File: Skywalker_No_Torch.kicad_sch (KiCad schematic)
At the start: 42 parts

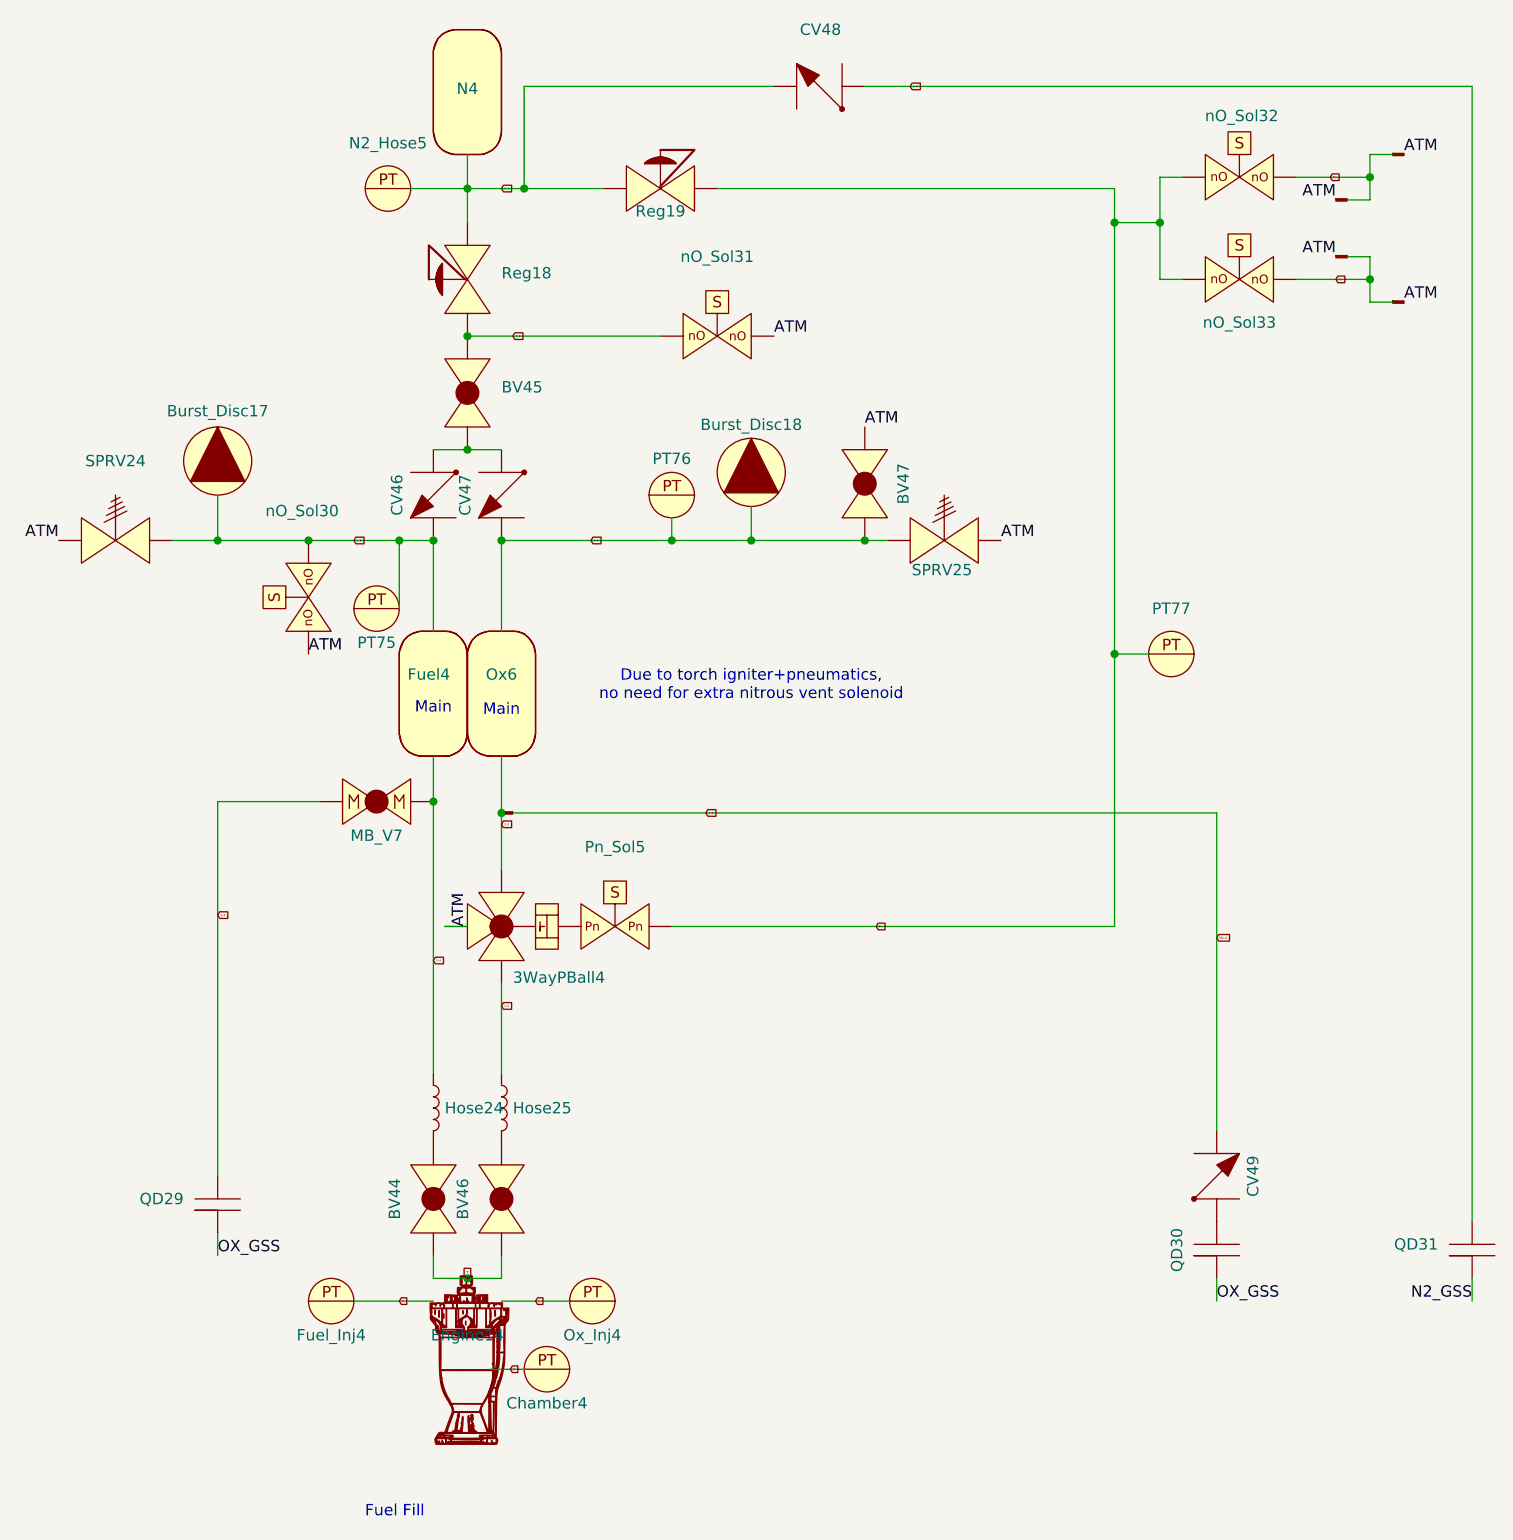
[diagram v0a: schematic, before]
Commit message: j0
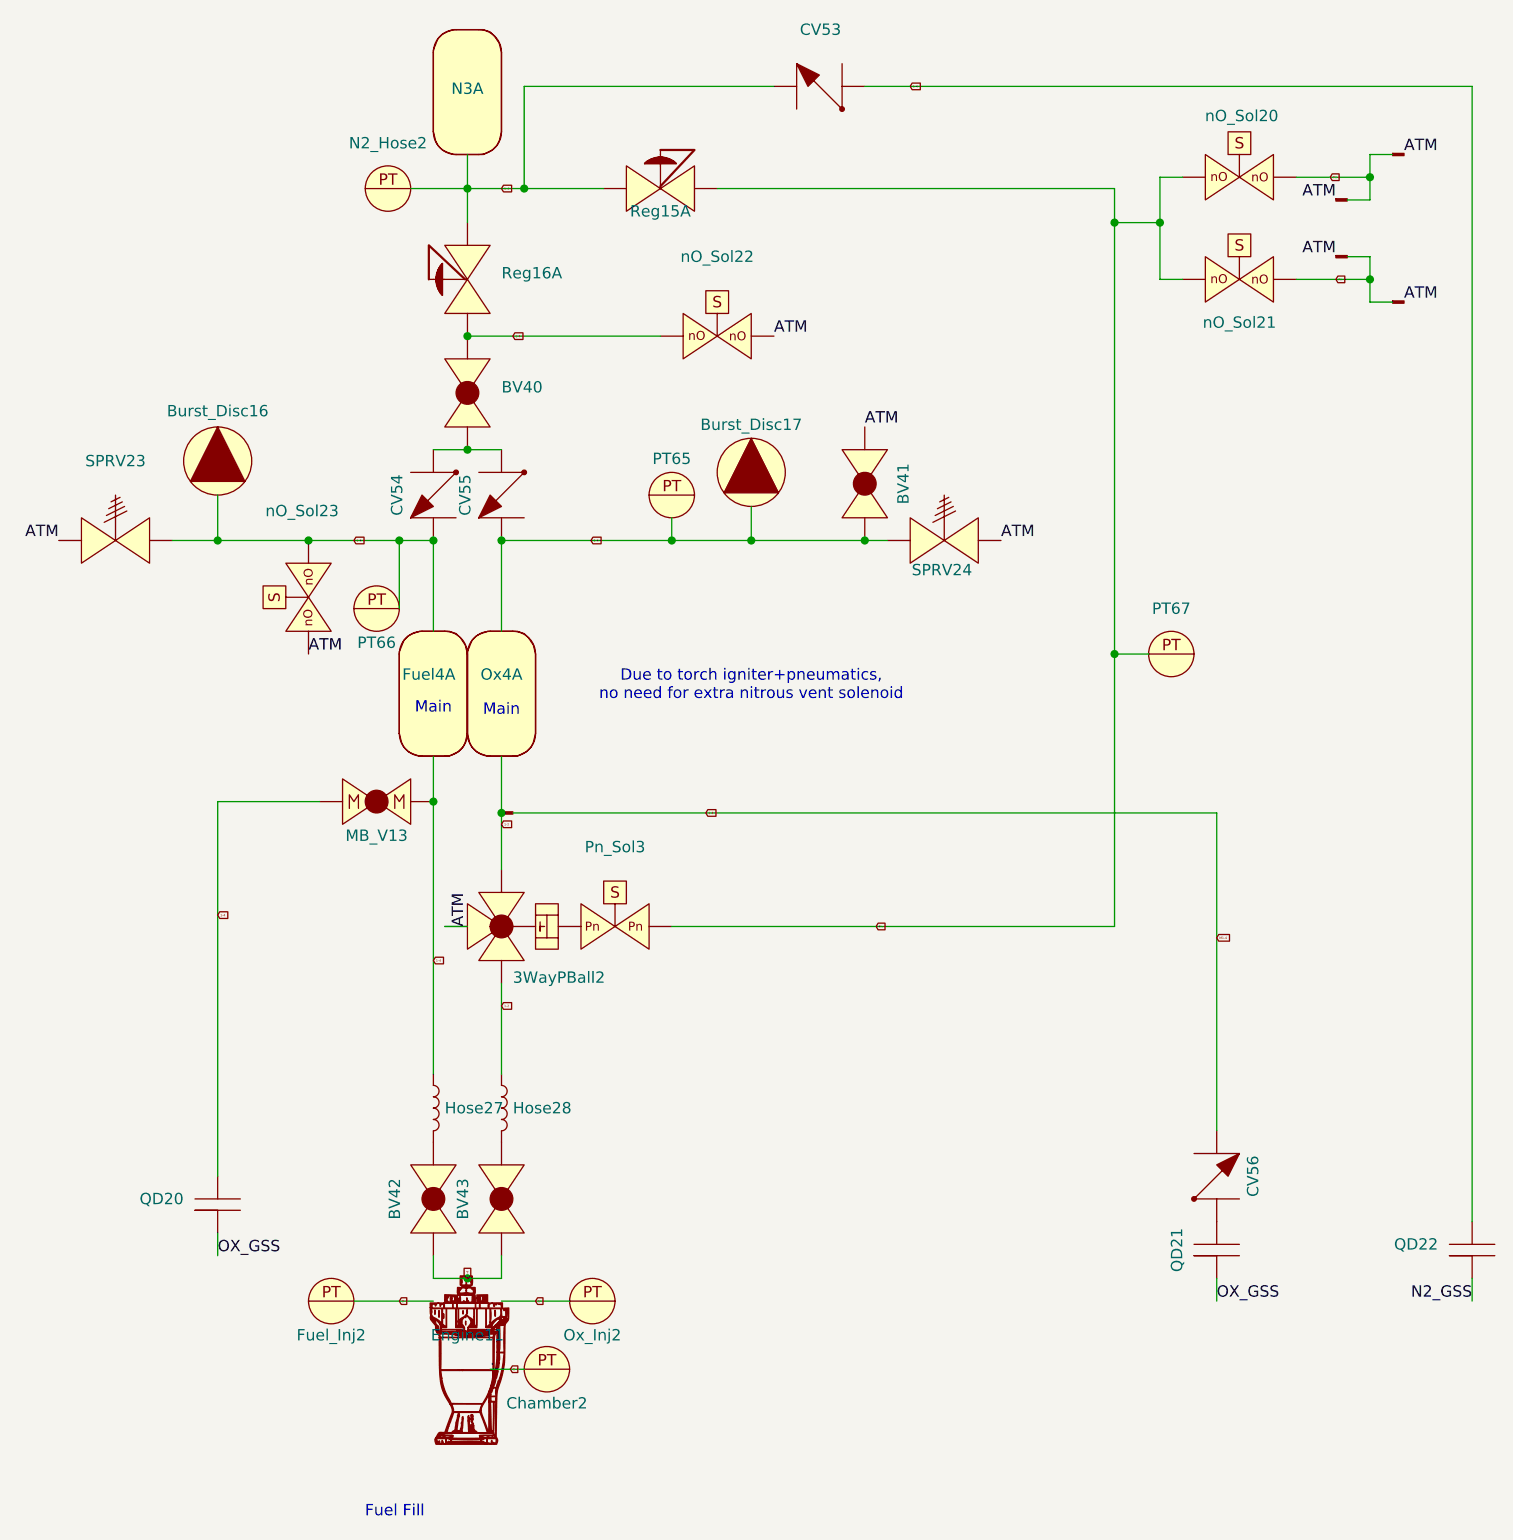
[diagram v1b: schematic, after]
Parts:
- renumbered 3WayPBall4 to 3WayPBall2, BV45 to BV40, BV47 to BV41, BV44 to BV42, BV46 to BV43, Burst_Disc17 to Burst_Disc16, Burst_Disc18 to Burst_Disc17, CV48 to CV53, CV46 to CV54, CV47 to CV55, CV49 to CV56, Chamber4 to Chamber2, Engine14 to Engine11, Fuel_Inj4 to Fuel_Inj2, Hose24 to Hose27, Hose25 to Hose28, MB_V7 to MB_V13, N2_Hose5 to N2_Hose2, N4 to N3, Ox6 to Ox4, Ox_Inj4 to Ox_Inj2, PT76 to PT65, PT75 to PT66, PT77 to PT67, Pn_Sol5 to Pn_Sol3, QD29 to QD20, QD30 to QD21, QD31 to QD22, Reg19 to Reg15, Reg18 to Reg16, SPRV24 to SPRV23, SPRV25 to SPRV24, U45 to U48, U46 to U49, U48 to U50, U44 to U51, nO_Sol32 to nO_Sol20, nO_Sol33 to nO_Sol21, nO_Sol31 to nO_Sol22, nO_Sol30 to nO_Sol23
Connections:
- new net: BV40., CV54., CV55.
- new net: CV56., QD21.
- new net: 3WayPBall2., Pn_Sol3.

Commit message: more silwood stuff
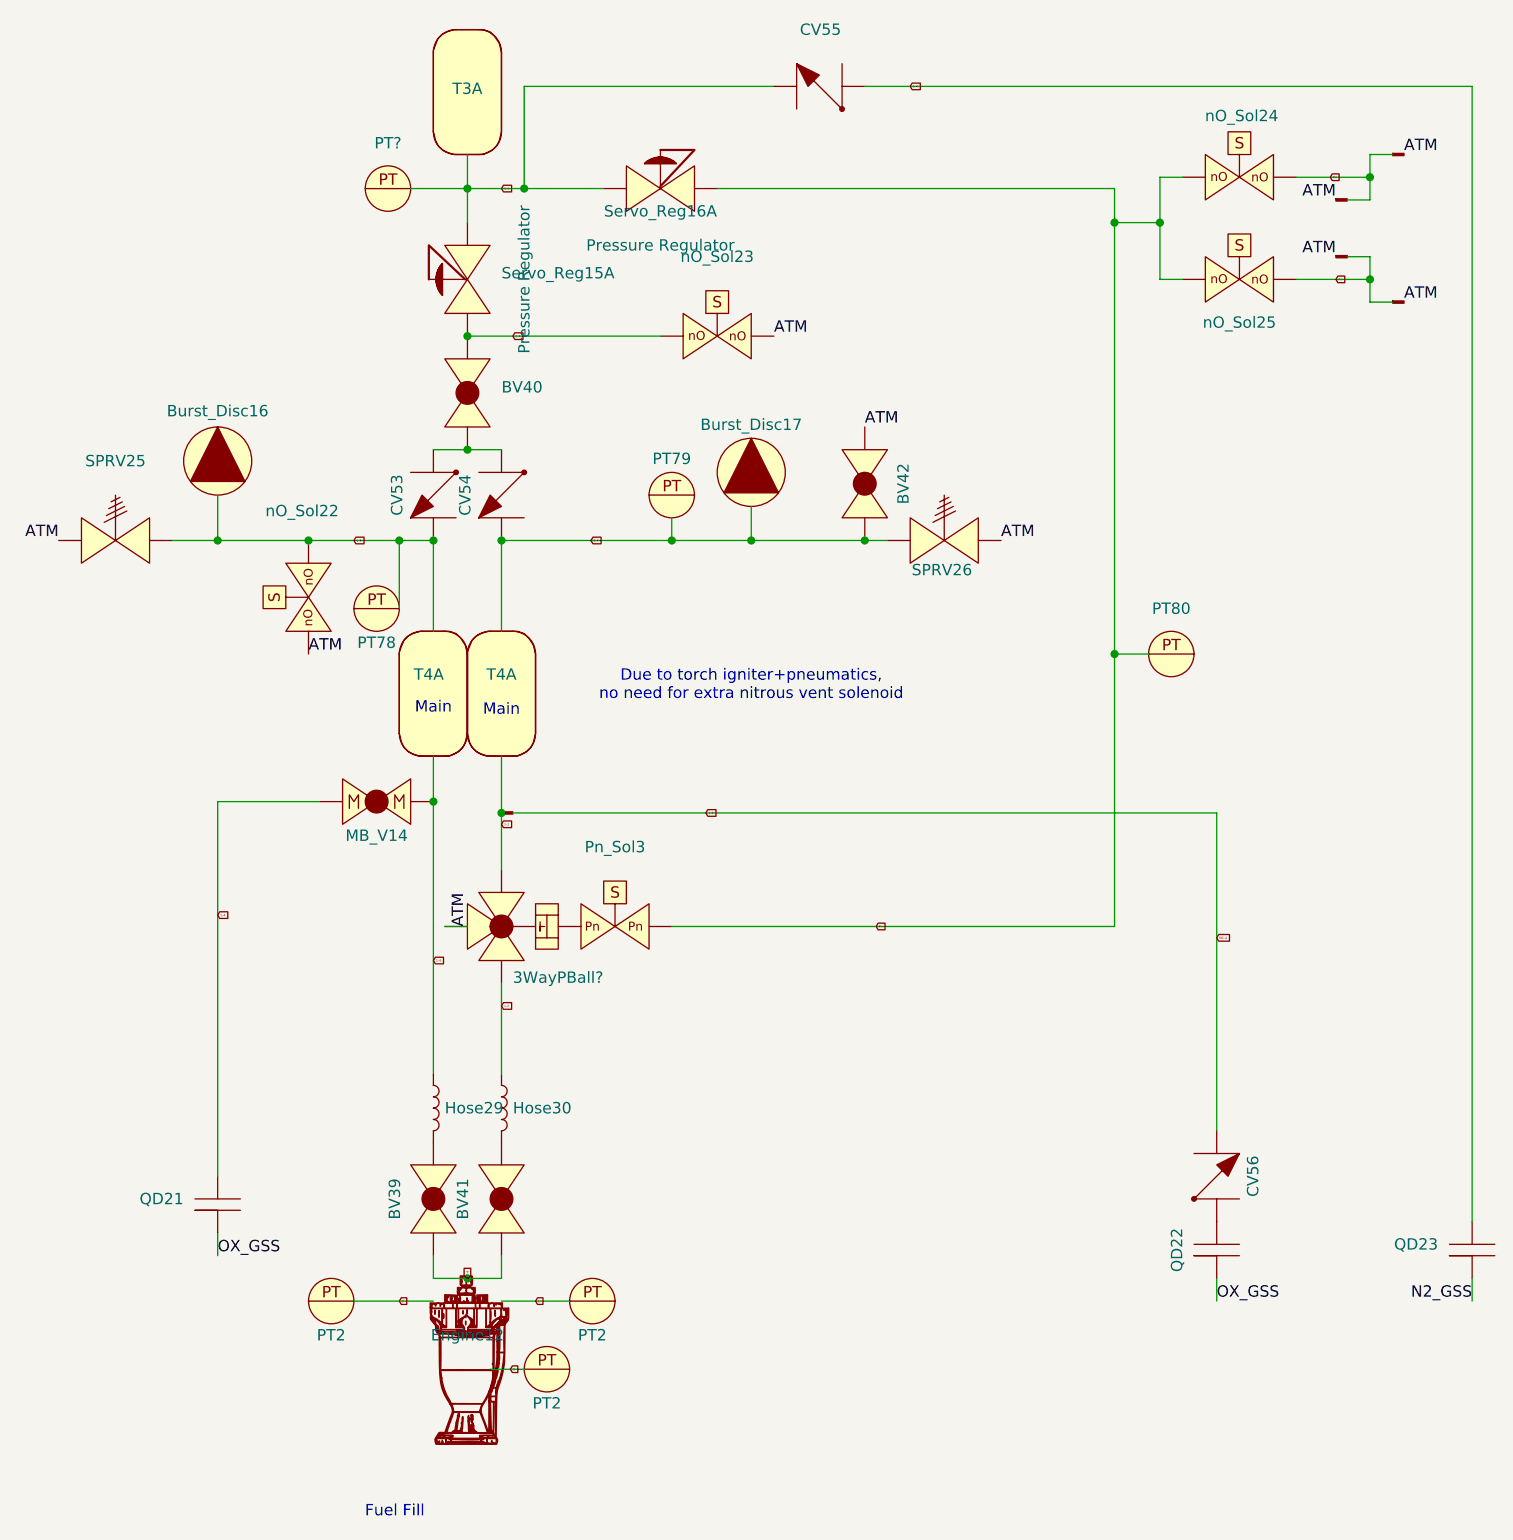
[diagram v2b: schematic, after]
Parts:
- renumbered 3WayPBall2 to 3WayPBall?, BV42 to BV39, BV43 to BV41, BV41 to BV42, CV54 to CV53, CV55 to CV54, CV53 to CV55, Engine11 to Engine12, Hose27 to Hose29, Hose28 to Hose30, MB_V13 to MB_V14, Chamber2 to PT2, Ox_Inj2 to PT2, Fuel_Inj2 to PT2, PT66 to PT78, PT65 to PT79, PT67 to PT80, N2_Hose2 to PT?, QD20 to QD21, QD21 to QD22, QD22 to QD23, SPRV23 to SPRV25, SPRV24 to SPRV26, Reg16 to Servo_Reg15, Reg15 to Servo_Reg16, N3 to T3, Fuel4 to T4, Ox4 to T4, U51 to U62, U48 to U63, U49 to U64, U47 to U65, U50 to U66, nO_Sol23 to nO_Sol22, nO_Sol22 to nO_Sol23, nO_Sol20 to nO_Sol24, nO_Sol21 to nO_Sol25
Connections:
- new net: BV40., CV53., CV54.
- new net: CV56., QD22.
- new net: 3WayPBall?., Pn_Sol3.

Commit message: Formatiing
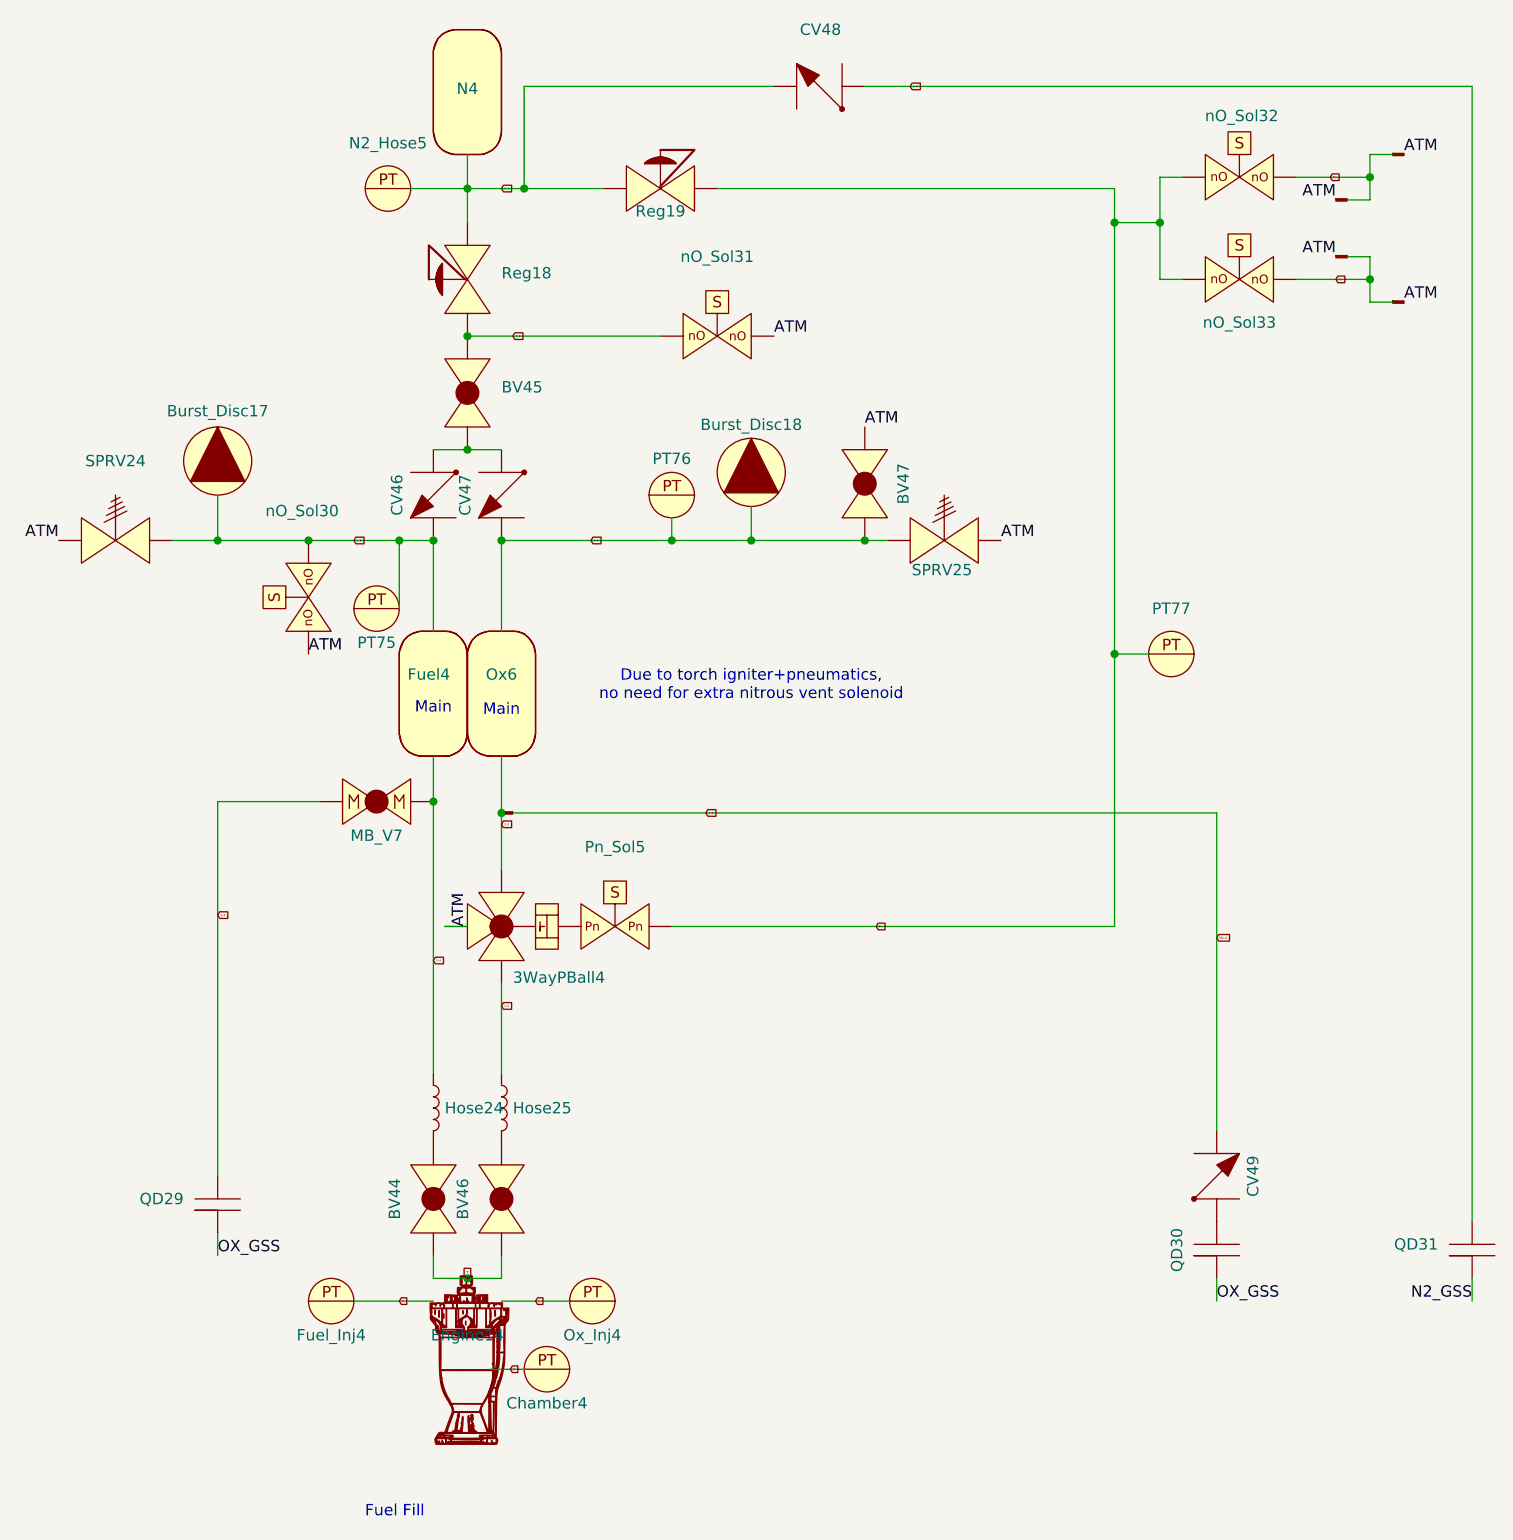
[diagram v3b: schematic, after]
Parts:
- gave numbers to parts that had none: 2
- renumbered BV39 to BV44, BV40 to BV45, BV41 to BV46, BV42 to BV47, Burst_Disc16 to Burst_Disc17, Burst_Disc17 to Burst_Disc18, CV53 to CV46, CV54 to CV47, CV55 to CV48, CV56 to CV49, PT2 to Chamber4, Engine12 to Engine14, T4 to Fuel4, PT2 to Fuel_Inj4, Hose29 to Hose24, Hose30 to Hose25, MB_V14 to MB_V7, T3 to N4, T4 to Ox6, PT2 to Ox_Inj4, PT78 to PT75, PT79 to PT76, PT80 to PT77, Pn_Sol3 to Pn_Sol5, QD21 to QD29, QD22 to QD30, QD23 to QD31, Servo_Reg15 to Reg18, Servo_Reg16 to Reg19, SPRV25 to SPRV24, SPRV26 to SPRV25, U62 to U44, U63 to U45, U64 to U46, U65 to U47, U66 to U48, nO_Sol22 to nO_Sol30, nO_Sol23 to nO_Sol31, nO_Sol24 to nO_Sol32, nO_Sol25 to nO_Sol33
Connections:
- new net: BV45., CV46., CV47.
- new net: CV49., QD30.
- new net: 3WayPBall4., Pn_Sol5.
